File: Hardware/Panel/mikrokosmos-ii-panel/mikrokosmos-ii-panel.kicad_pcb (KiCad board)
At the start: 2 copper layers, 25 x 200 mm, 9 parts

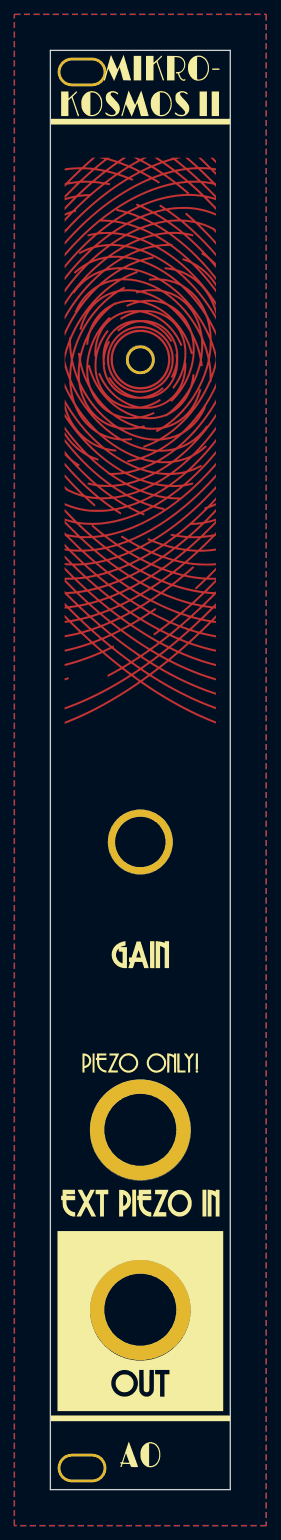
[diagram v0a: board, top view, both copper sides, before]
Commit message: panel, PCB updates
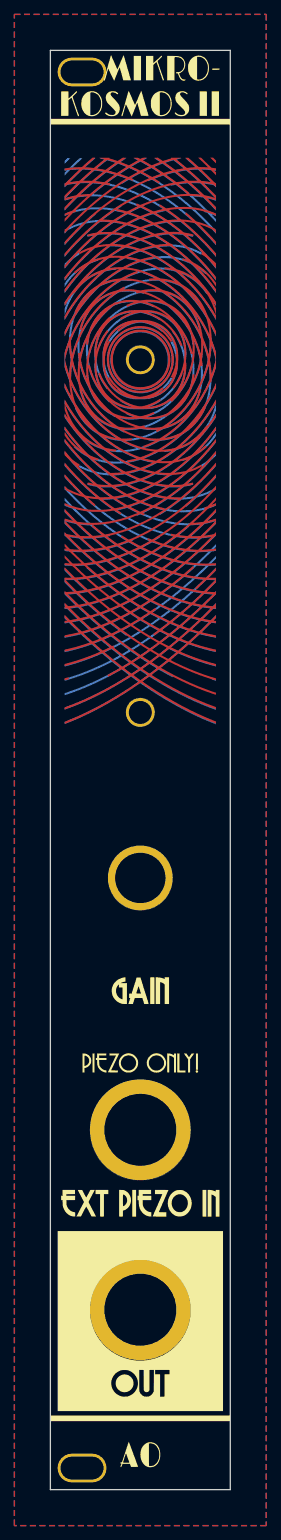
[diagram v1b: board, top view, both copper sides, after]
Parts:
- added GRAF5: Art inverted, mikrokosmos-ii-panel:mikrokosmos-ii_panel_inv_art, B.Cu at (28.6, 107.7)
- added H6: Mounting_Hole, Kosmo_panel:Kosmo_Panel_Mounting_Hole, F.Cu at (28.6, 99.6)
- GRAF1: footprint mikrokosmos-ii-panel:mikrokosmos-ii-panel-holes -> mikrokosmos-ii-panel:mikrokosmos-ii_panel_holes
- GRAF2: footprint mikrokosmos-ii-panel:mikrokosmos-ii-panel-art -> mikrokosmos-ii-panel:mikrokosmos-ii_panel_art
- GRAF3: value CC0 logo -> Art for Cu; footprint ao_tht:CC0_logo -> mikrokosmos-ii-panel:mikrokosmos-ii_panel_artc
- GRAF4: footprint mikrokosmos-ii-panel:mikrokosmos-ii-panel-artc -> mikrokosmos-ii-panel:mikrokosmos-ii_panel_artc
- moved GRAF3 150.0 mm to (28.6, 52.6)
- moved H4 5.00 mm to (28.6, 122.6)
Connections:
- H3 pad 1: GND -> unconnected-(H3-Pad1)
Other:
- board text removed: "Panel design by Rich Holmes CC0 1.0 7/2022 JLCJLCJLCJLC"
